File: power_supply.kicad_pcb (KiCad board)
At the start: 2 copper layers, 144.8 x 50.8 mm, 19 parts

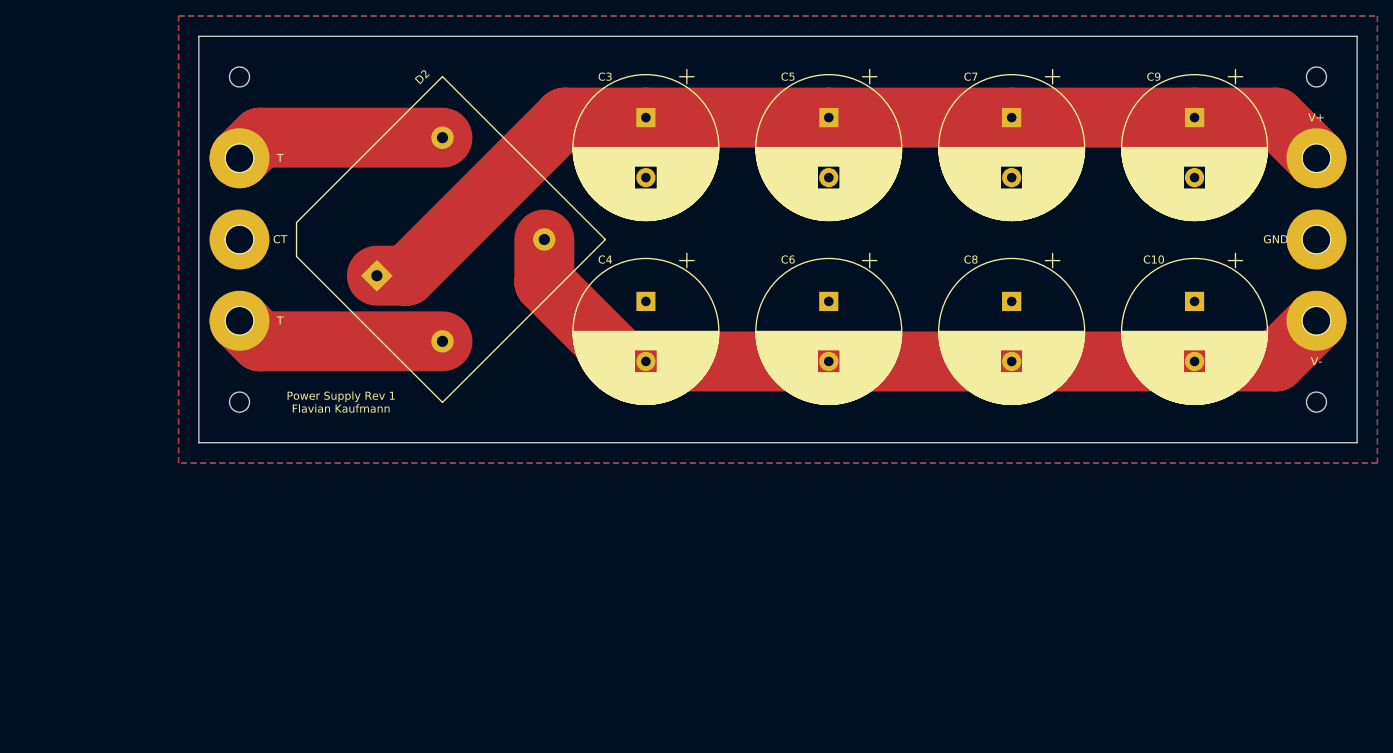
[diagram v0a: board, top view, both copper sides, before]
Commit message: cosmetics
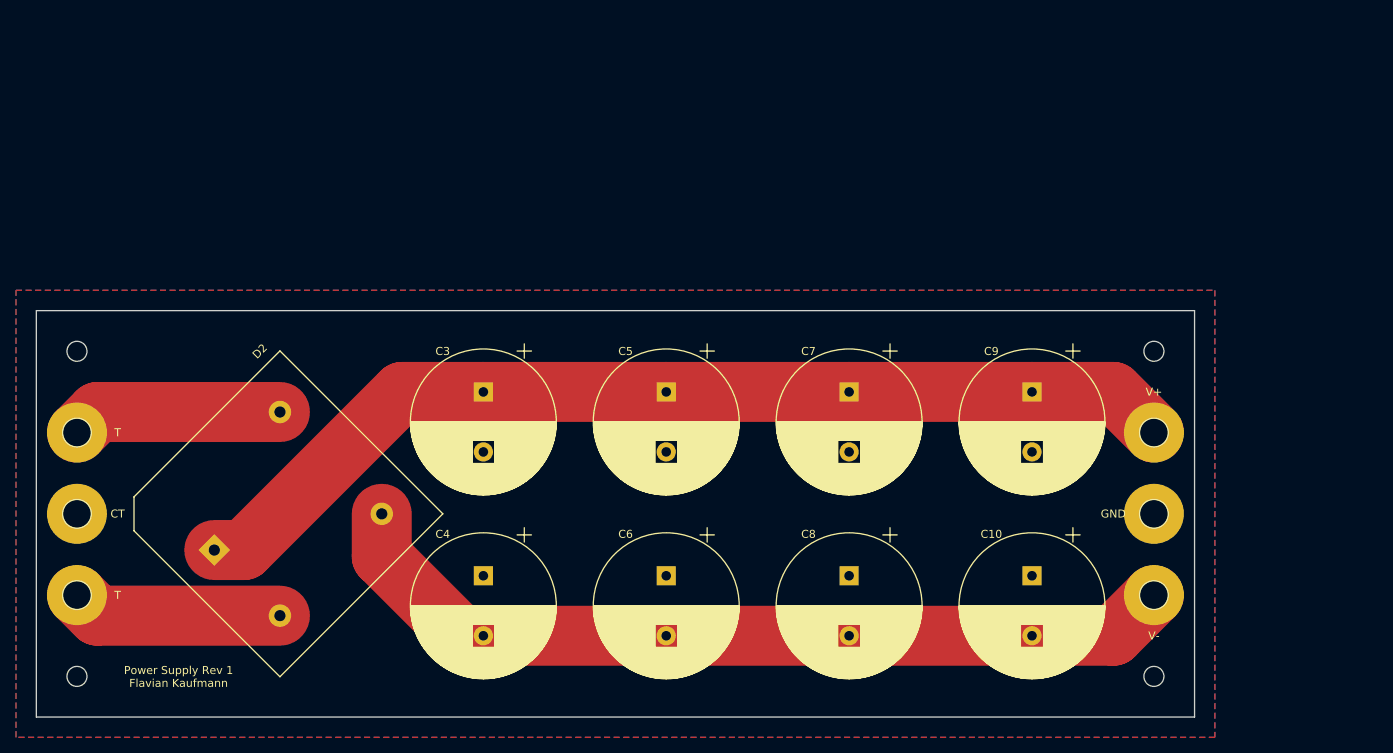
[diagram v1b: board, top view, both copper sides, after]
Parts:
- moved C3 39.9 mm to (127.0, 80.0)
- moved C5 39.9 mm to (149.9, 80.0)
- moved C7 39.9 mm to (172.7, 80.0)
- moved C9 39.9 mm to (195.6, 80.0)
- moved D2 39.9 mm to (93.4, 99.8)
- moved REF** 39.9 mm to (76.2, 85.1)
- moved REF** 39.9 mm to (210.8, 85.1)
- moved REF** 39.9 mm to (210.8, 74.9)
- moved REF** 39.9 mm to (76.2, 74.9)
- moved REF** 39.9 mm to (210.8, 95.2)
- moved REF** 39.9 mm to (76.2, 95.2)
- moved C10 39.9 mm to (195.6, 103.0)
- moved C4 39.9 mm to (127.0, 103.0)
- moved C6 39.9 mm to (149.9, 103.0)
- moved C8 39.9 mm to (172.7, 103.0)
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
